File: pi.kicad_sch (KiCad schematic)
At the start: 3 parts, among them J33 2540-5

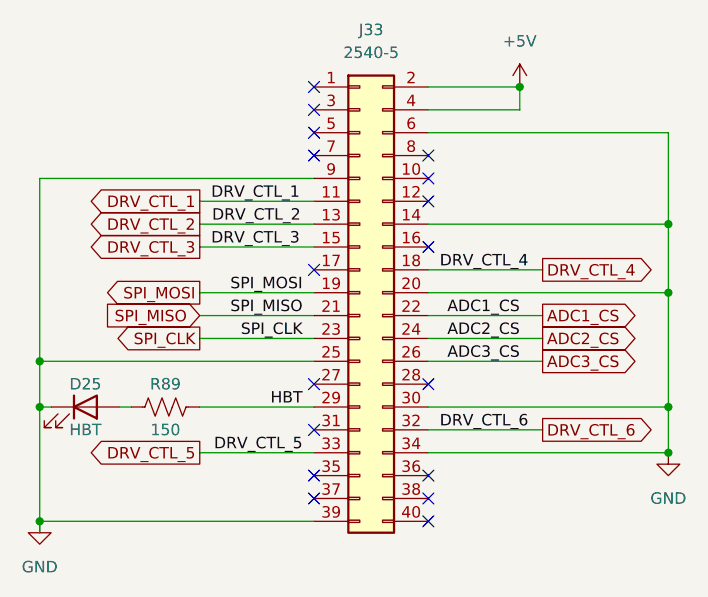
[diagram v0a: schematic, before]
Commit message: some minor schematic cleanup
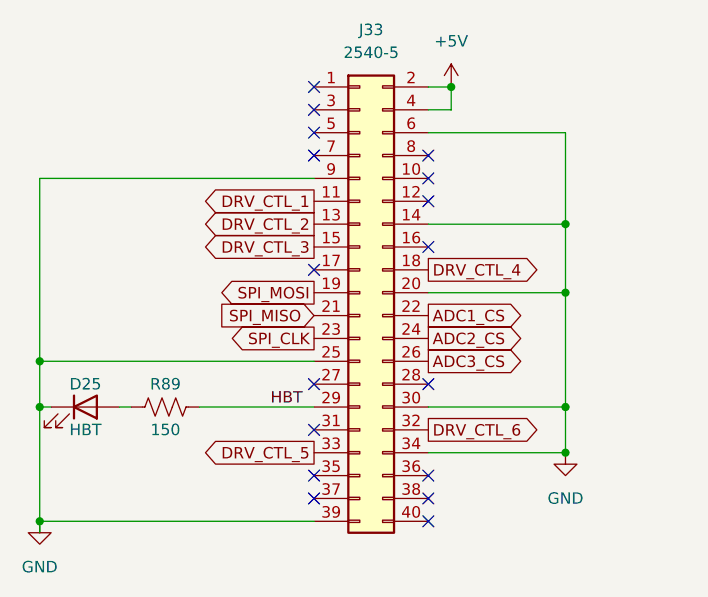
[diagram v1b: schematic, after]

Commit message: shuffle around some parts
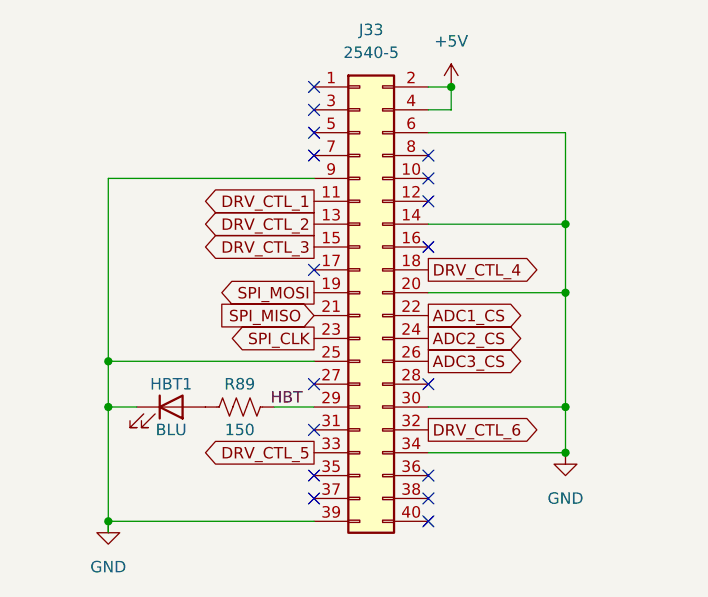
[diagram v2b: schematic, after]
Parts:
- HBT1: renamed from D25; value HBT -> BLU
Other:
- moved on the sheet: HBT1, R89
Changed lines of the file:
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@@
     (company "Rice Eclipse")
   )
-  (junction (at 68.58 92.71) (diameter 0) (color 0 0 0 0)
+  (junction (at 76.2 92.71) (diameter 0) (color 0 0 0 0)
   )
   (junction (at 127 97.79) (diameter 0) (color 0 0 0 0)
@@
   (junction (at 114.3 62.23) (diameter 0) (color 0 0 0 0)
   )
-  (junction (at 68.58 97.79) (diameter 0) (color 0 0 0 0)
+  (junction (at 76.2 97.79) (diameter 0) (color 0 0 0 0)
   )
   (junction (at 127 77.47) (diameter 0) (color 0 0 0 0)
   )
-  (junction (at 68.58 110.49) (diameter 0) (color 0 0 0 0)
+  (junction (at 76.2 110.49) (diameter 0) (color 0 0 0 0)
   )
   (junction (at 127 85.09) (diameter 0) (color 0 0 0 0)
@@
     (stroke (width 0) (type default) (color 0 0 0 0))
   )
-  (wire (pts (xy 68.58 110.49) (xy 68.58 111.76))
+  (wire (pts (xy 76.2 110.49) (xy 76.2 111.76))
     (stroke (width 0) (type default) (color 0 0 0 0))
   )
@@
     (stroke (width 0) (type default) (color 0 0 0 0))
   )
-  (wire (pts (xy 77.47 97.79) (xy 78.74 97.79))
-    (stroke (width 0) (type default) (color 0 0 0 0))
-  )
-  (wire (pts (xy 68.58 72.39) (xy 99.06 72.39))
-    (stroke (width 0) (type default) (color 0 0 0 0))
-  )
-  (wire (pts (xy 68.58 110.49) (xy 99.06 110.49))
+  (wire (pts (xy 76.2 72.39) (xy 99.06 72.39))
+    (stroke (width 0) (type default) (color 0 0 0 0))
+  )
+  (wire (pts (xy 76.2 110.49) (xy 99.06 110.49))
     (stroke (width 0) (type default) (color 0 0 0 0))
   )
@@
     (stroke (width 0) (type default) (color 0 0 0 0))
   )
-  (wire (pts (xy 68.58 97.79) (xy 69.85 97.79))
+  (wire (pts (xy 76.2 97.79) (xy 79.375 97.79))
     (stroke (width 0) (type default) (color 0 0 0 0))
   )
@@
     (stroke (width 0) (type default) (color 0 0 0 0))
   )
-  (wire (pts (xy 68.58 92.71) (xy 99.06 92.71))
-    (stroke (width 0) (type default) (color 0 0 0 0))
-  )
-  (wire (pts (xy 68.58 97.79) (xy 68.58 110.49))
+  (wire (pts (xy 76.2 92.71) (xy 99.06 92.71))
+    (stroke (width 0) (type default) (color 0 0 0 0))
+  )
+  (wire (pts (xy 76.2 97.79) (xy 76.2 110.49))
     (stroke (width 0) (type default) (color 0 0 0 0))
   )
@@
     (stroke (width 0) (type default) (color 0 0 0 0))
   )
-  (wire (pts (xy 86.36 97.79) (xy 99.06 97.79))
+  (wire (pts (xy 94.615 97.79) (xy 99.06 97.79))
     (stroke (width 0) (type default) (color 0 0 0 0))
   )
@@
     (stroke (width 0) (type default) (color 0 0 0 0))
   )
-  (wire (pts (xy 68.58 72.39) (xy 68.58 92.71))
-    (stroke (width 0) (type default) (color 0 0 0 0))
-  )
-  (wire (pts (xy 68.58 92.71) (xy 68.58 97.79))
+  (wire (pts (xy 76.2 72.39) (xy 76.2 92.71))
+    (stroke (width 0) (type default) (color 0 0 0 0))
+  )
+  (wire (pts (xy 76.2 92.71) (xy 76.2 97.79))
     (stroke (width 0) (type default) (color 0 0 0 0))
   )
@@
     (pin "1")
   )
-  (symbol (lib_id "power:GND") (at 68.58 110.49 0) (unit 1)
-    (in_bom yes) (on_board yes) (fields_autoplaced)
-    (property "Reference" "#PWR0154" (id 0) (at 68.58 116.84 0)
-      (effects (font (size 1.27 1.27)) hide)
-    )
-    (property "Value" "GND" (id 1) (at 68.58 115.57 0))
-    (property "Footprint" "" (id 2) (at 68.58 110.49 0)
-      (effects (font (size 1.27 1.27)) hide)
-    )
-    (property "Datasheet" "" (id 3) (at 68.58 110.49 0)
-      (effects (font (size 1.27 1.27)) hide)
-    )
-    (pin "1")
-  )
-  (symbol (lib_id "Device:R_US") (at 82.55 97.79 90) (unit 1)
+  (symbol (lib_id "power:GND") (at 76.2 110.49 0) (unit 1)
+    (in_bom yes) (on_board yes) (fields_autoplaced)
+    (property "Reference" "#PWR0154" (id 0) (at 76.2 116.84 0)
+      (effects (font (size 1.27 1.27)) hide)
+    )
+    (property "Value" "GND" (id 1) (at 76.2 115.57 0))
+    (property "Footprint" "" (id 2) (at 76.2 110.49 0)
+      (effects (font (size 1.27 1.27)) hide)
+    )
+    (property "Datasheet" "" (id 3) (at 76.2 110.49 0)
+      (effects (font (size 1.27 1.27)) hide)
+    )
+    (pin "1")
+  )
+  (symbol (lib_id "Device:R_US") (at 90.805 97.79 90) (unit 1)
     (in_bom yes) (on_board yes)
-    (property "Reference" "R89" (id 0) (at 82.55 95.25 90))
-    (property "Value" "150" (id 1) (at 82.55 100.33 90))
-    (property "Footprint" "Resistor_SMD:R_1206_3216Metric" (id 2) (at 82.804 96.774 90)
-      (effects (font (size 1.27 1.27)) hide)
-    )
-    (property "Datasheet" "~" (id 3) (at 82.55 97.79 0)
+    (property "Reference" "R89" (id 0) (at 90.805 95.25 90))
+    (property "Value" "150" (id 1) (at 90.805 100.33 90))
+    (property "Footprint" "Resistor_SMD:R_1206_3216Metric" (id 2) (at 91.059 96.774 90)
+      (effects (font (size 1.27 1.27)) hide)
+    )
+    (property "Datasheet" "~" (id 3) (at 90.805 97.79 0)
       (effects (font (size 1.27 1.27)) hide)
     )
@@
     (pin "9")
   )
-  (symbol (lib_id "Device:LED") (at 73.66 97.79 0) (unit 1)
+  (symbol (lib_id "Device:LED") (at 83.185 97.79 0) (unit 1)
     (in_bom yes) (on_board yes)
-    (property "Reference" "D25" (id 0) (at 73.66 95.25 0))
-    (property "Value" "HBT" (id 1) (at 73.66 100.33 0))
-    (property "Footprint" "LED_SMD:LED_1206_3216Metric" (id 2) (at 73.66 97.79 0)
-      (effects (font (size 1.27 1.27)) hide)
-    )
-    (property "Datasheet" "~" (id 3) (at 73.66 97.79 0)
-      (effects (font (size 1.27 1.27)) hide)
-    )
+    (property "Reference" "HBT1" (id 0) (at 83.185 95.25 0))
+    (property "Value" "BLU" (id 1) (at 83.185 100.33 0))
+    (property "Footprint" "LED_SMD:LED_1206_3216Metric" (id 2) (at 83.185 97.79 0)
+      (effects (font (size 1.27 1.27)) hide)
+    )
+    (property "Datasheet" "~" (id 3) (at 83.185 97.79 0)
+      (effects (font (size 1.27 1.27)) hide)
+    )
